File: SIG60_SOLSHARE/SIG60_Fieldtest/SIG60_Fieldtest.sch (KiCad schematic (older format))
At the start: 2 parts, among them U1 PLC_BOARD

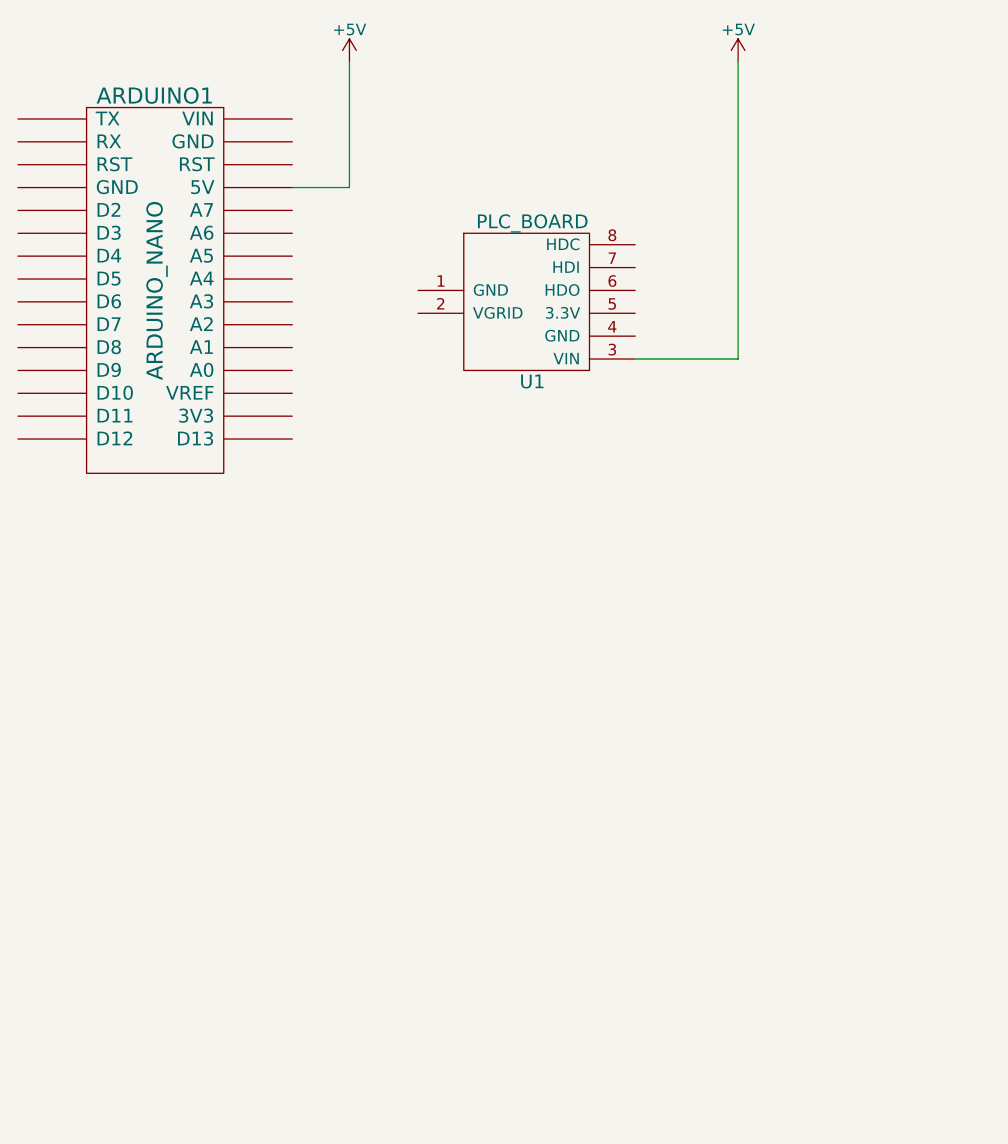
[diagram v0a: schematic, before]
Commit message: cleanup before further PLC development
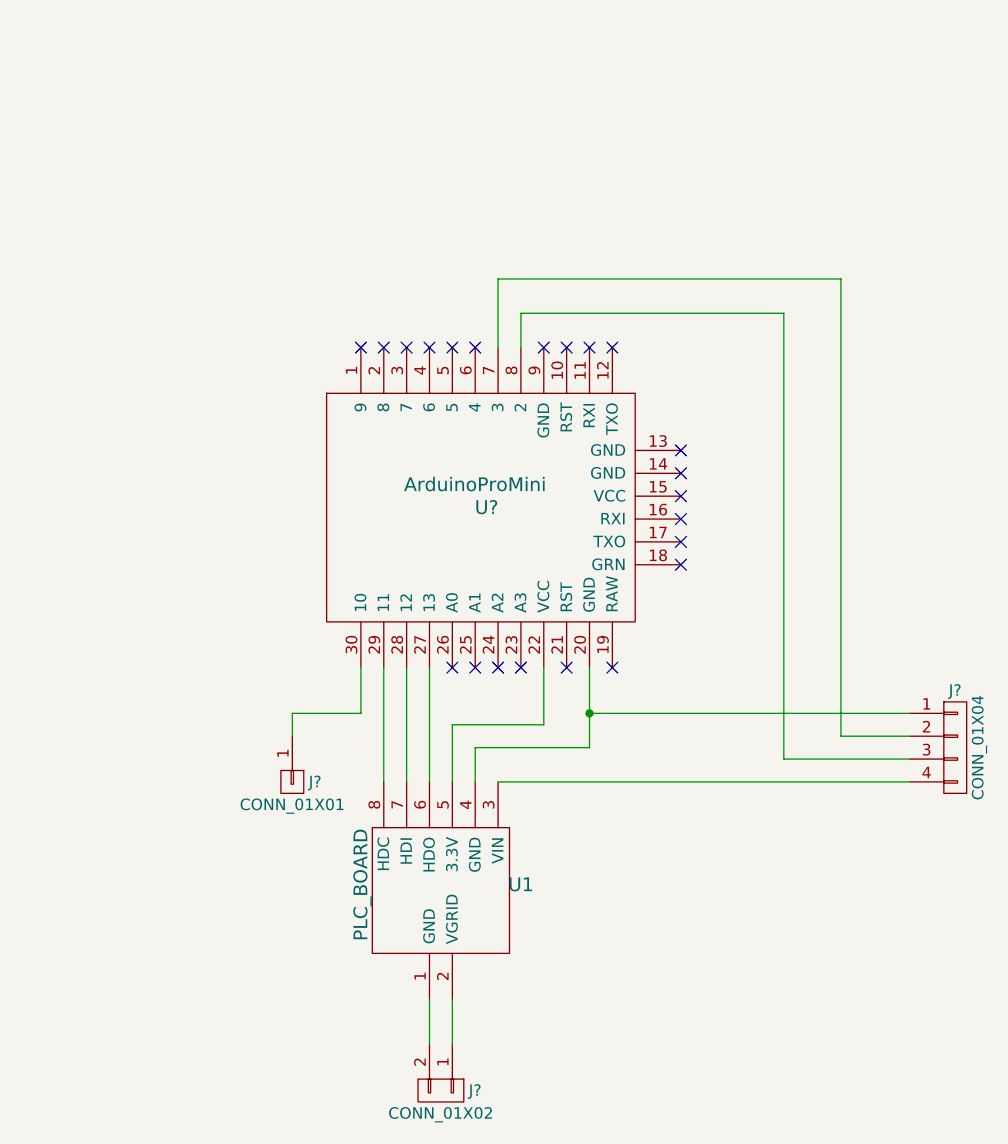
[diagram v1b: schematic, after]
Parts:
- removed ARDUINO1: ARDUINO_NANO, Modules:Arduino_Nano, symbol ARDUINO_NANO
- added J?: CONN_01X02, symbol CONN_01X02
- added J?: CONN_01X04, symbol CONN_01X04
- added J?: CONN_01X01, symbol CONN_01X01
- added U?: ArduinoProMini, symbol ArduinoProMini
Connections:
- net at U1.1 (GND): now also J?.2 (P2)
- net at U1.2 (VGRID): now also J?.1 (P1)
- net at U1.4 (GND): now also J?.1 (P1), U?.20 (GND)
- net at U1.5 (3.3V): now also U?.22 (VCC)
- net at U1.6 (HDO): now also U?.27 (13)
- net at U1.7 (HDI): now also U?.28 (12)
- net at U1.8 (HDC): now also U?.29 (11)
- net +5V: no longer names the net of U1.3 (VIN)
- net +5V: now also J?.4 (P4)
- new net: J?.1 (P1), U?.30 (10)
- new net: J?.2 (P2), U?.7 (3)
- new net: J?.3 (P3), U?.8 (2)
- no-connect marks 0 -> 22
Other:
- moved on the sheet: U1
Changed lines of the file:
@@
 $EndDescr
 $Comp
-L ARDUINO_NANO ARDUINO1
-U 1 1 5A3D0EC5
-P 2100 1950
-F 0 "ARDUINO1" H 2100 2800 70  0000 C CNN
-F 1 "ARDUINO_NANO" V 2100 1950 70  0000 C CNN
-F 2 "Modules:Arduino_Nano" H 2100 1950 60  0001 C CNN
-F 3 "" H 2100 1950 60  0000 C CNN
-	1    2100 1950
+L PLC_BOARD U1
+U 1 1 5A3BAFAB
+P 3350 4550
+F 0 "U1" V 3350 4200 60  0000 C CNN
+F 1 "PLC_BOARD" H 3350 4900 60  0000 C CNN
+F 2 ".pretty:PLC_BOARD" H 3350 4550 60  0001 C CNN
+F 3 "" H 3350 4550 60  0001 C CNN
+	1    3350 4550
+	0    -1   -1   0
+$EndComp
+$Comp
+L ArduinoProMini U?
+U 1 1 5A5607D3
+P 3550 2900
+F 0 "U?" H 3550 2900 60  0000 C CNN
+F 1 "ArduinoProMini" H 3500 3000 60  0000 C CNN
+F 2 "" H 3550 2900 60  0001 C CNN
+F 3 "" H 3550 2900 60  0001 C CNN
+	1    3550 2900
 	1    0    0    -1
 $EndComp
 $Comp
-L PLC_BOARD U1
-U 1 1 5A3BAFAB
-P 3750 2000
-F 0 "U1" H 3750 1650 60  0000 C CNN
-F 1 "PLC_BOARD" H 3750 2350 60  0000 C CNN
-F 2 ".pretty:PLC_BOARD" H 3750 2000 60  0001 C CNN
-F 3 "" H 3750 2000 60  0001 C CNN
-	1    3750 2000
-	1    0    0    -1
+L CONN_01X02 J?
+U 1 1 5A561214
+P 3350 5450
+F 0 "J?" V 3350 5600 50  0000 C CNN
+F 1 "CONN_01X02" V 3450 5450 50  0000 C CNN
+F 2 "" H 3350 5450 50  0001 C CNN
+F 3 "" H 3350 5450 50  0001 C CNN
+	1    3350 5450
+	0    1    1    0
 $EndComp
+NoConn ~ 3000 2200
+NoConn ~ 3100 2200
+NoConn ~ 3200 2200
+NoConn ~ 3300 2200
+NoConn ~ 3400 2200
+NoConn ~ 3500 2200
+NoConn ~ 3900 2200
+NoConn ~ 4000 2200
+NoConn ~ 4100 2200
+NoConn ~ 4400 2650
+NoConn ~ 4400 3150
+NoConn ~ 4100 3600
+NoConn ~ 3900 3600
+NoConn ~ 3700 3600
+NoConn ~ 3600 3600
+NoConn ~ 3500 3600
+NoConn ~ 3400 3600
 $Comp
-L +5V #PWR?
-U 1 1 5A3BB8FE
-P 2950 950
-F 0 "#PWR?" H 2950 800 50  0001 C CNN
-F 1 "+5V" H 2950 1090 50  0000 C CNN
-F 2 "" H 2950 950 50  0001 C CNN
-F 3 "" H 2950 950 50  0001 C CNN
-	1    2950 950
+L CONN_01X04 J?
+U 1 1 5A5793DC
+P 5600 3950
+F 0 "J?" H 5600 4200 50  0000 C CNN
+F 1 "CONN_01X04" V 5700 3950 50  0000 C CNN
+F 2 "" H 5600 3950 50  0001 C CNN
+F 3 "" H 5600 3950 50  0001 C CNN
+	1    5600 3950
 	1    0    0    -1
 $EndComp
 Wire Wire Line
-	2950 950  2950 1500
+	3300 5250 3300 5050
 Wire Wire Line
-	2950 1500 2700 1500
+	3400 5250 3400 5050
+Wire Wire Line
+	3100 3600 3100 4100
+Wire Wire Line
+	3200 3600 3200 4100
+Wire Wire Line
+	3300 3600 3300 4100
+Wire Wire Line
+	3400 4100 3400 3850
+Wire Wire Line
+	3400 3850 3800 3850
+Wire Wire Line
+	3800 3850 3800 3600
+Wire Wire Line
+	4000 3600 4000 3950
+Wire Wire Line
+	4000 3800 5400 3800
+Wire Wire Line
+	3600 4100 5400 4100
+Wire Wire Line
+	3500 4100 3500 3950
+Wire Wire Line
+	3500 3950 4000 3950
+Connection ~ 4000 3800
+NoConn ~ 4400 3050
+NoConn ~ 4400 2950
+NoConn ~ 4400 2850
+NoConn ~ 4400 2750
+Wire Wire Line
+	5400 3900 5100 3900
+Wire Wire Line
+	5100 3900 5100 1900
+Wire Wire Line
+	5100 1900 3600 1900
+Wire Wire Line
+	3600 1900 3600 2200
+Wire Wire Line
+	5400 4000 4850 4000
+Wire Wire Line
+	4850 4000 4850 2050
+Wire Wire Line
+	4850 2050 3700 2050
+Wire Wire Line
+	3700 2050 3700 2200
+NoConn ~ 3800 2200
 $Comp
-L +5V #PWR?
-U 1 1 5A3BB97E
-P 4650 950
-F 0 "#PWR?" H 4650 800 50  0001 C CNN
-F 1 "+5V" H 4650 1090 50  0000 C CNN
-F 2 "" H 4650 950 50  0001 C CNN
-F 3 "" H 4650 950 50  0001 C CNN
-	1    4650 950
-	1    0    0    -1
+L CONN_01X01 J?
+U 1 1 5A5C9B55
+P 2700 4100
+F 0 "J?" V 2700 4200 50  0000 C CNN
+F 1 "CONN_01X01" V 2800 4100 50  0000 C CNN
+F 2 "" H 2700 4100 50  0001 C CNN
+F 3 "" H 2700 4100 50  0001 C CNN
+	1    2700 4100
+	0    1    1    0
 $EndComp
 Wire Wire Line
-	4200 2250 4650 2250
+	3000 3600 3000 3800
 Wire Wire Line
-	4650 2250 4650 950
+	3000 3800 2700 3800
+Wire Wire Line
+	2700 3800 2700 3900
 $EndSCHEMATC
